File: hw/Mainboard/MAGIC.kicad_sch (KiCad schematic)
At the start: 21 parts, among them SW1 RESET, SW4 NMI, U18 SN74LVC4245APWR, U19 SN74LVC4245APWR, U20 SN74LVC4245APWR

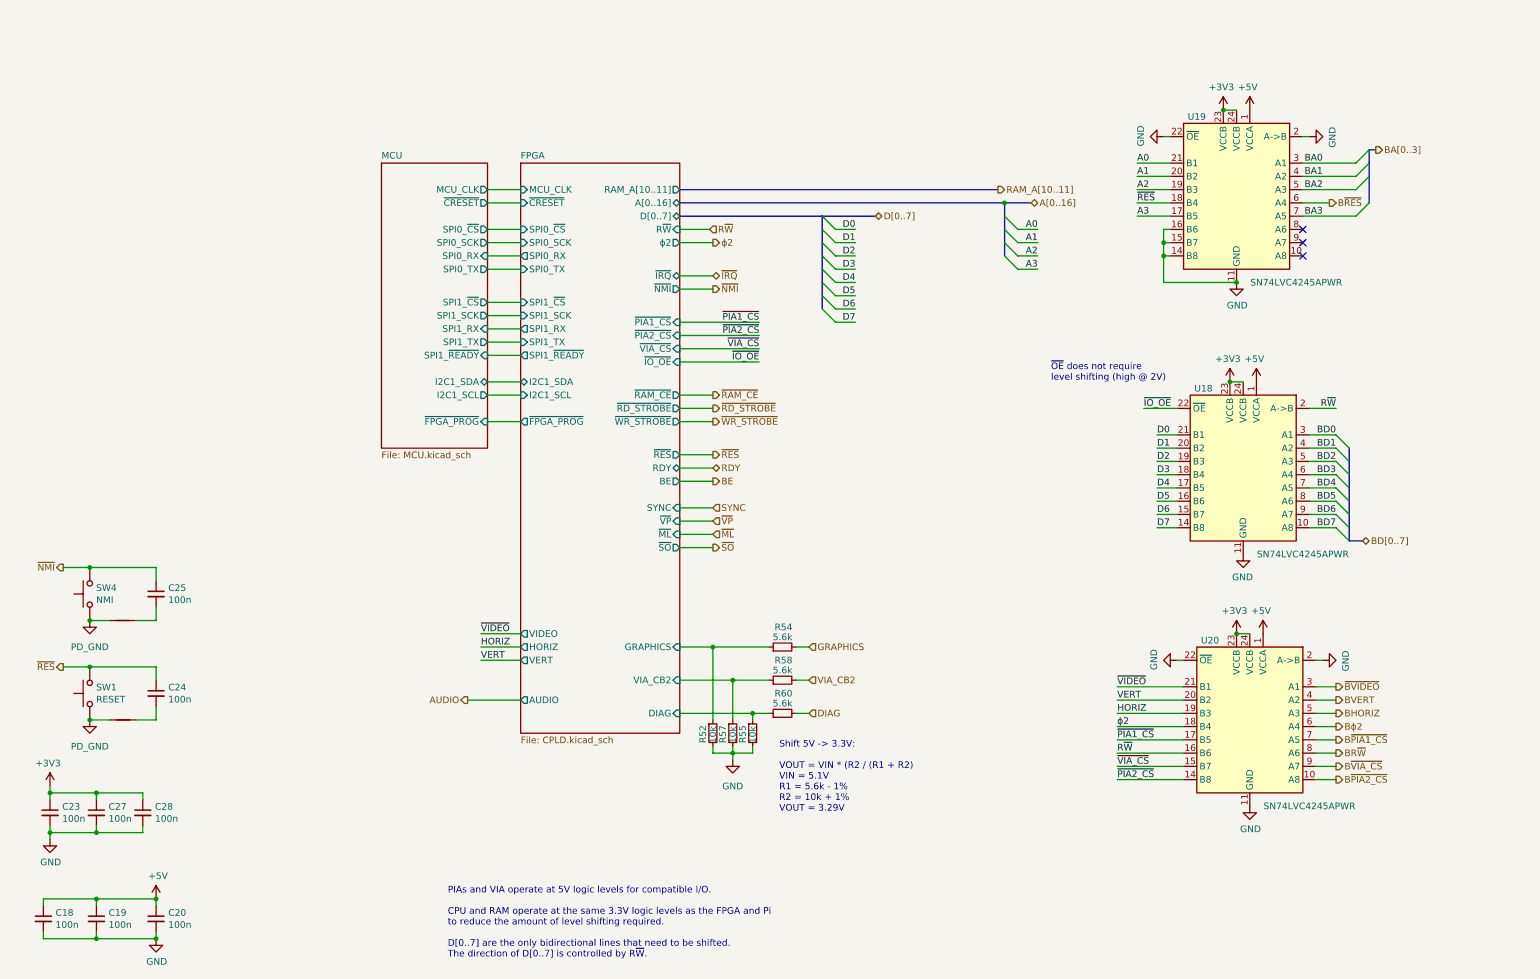
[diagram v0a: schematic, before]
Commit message: hw: wip
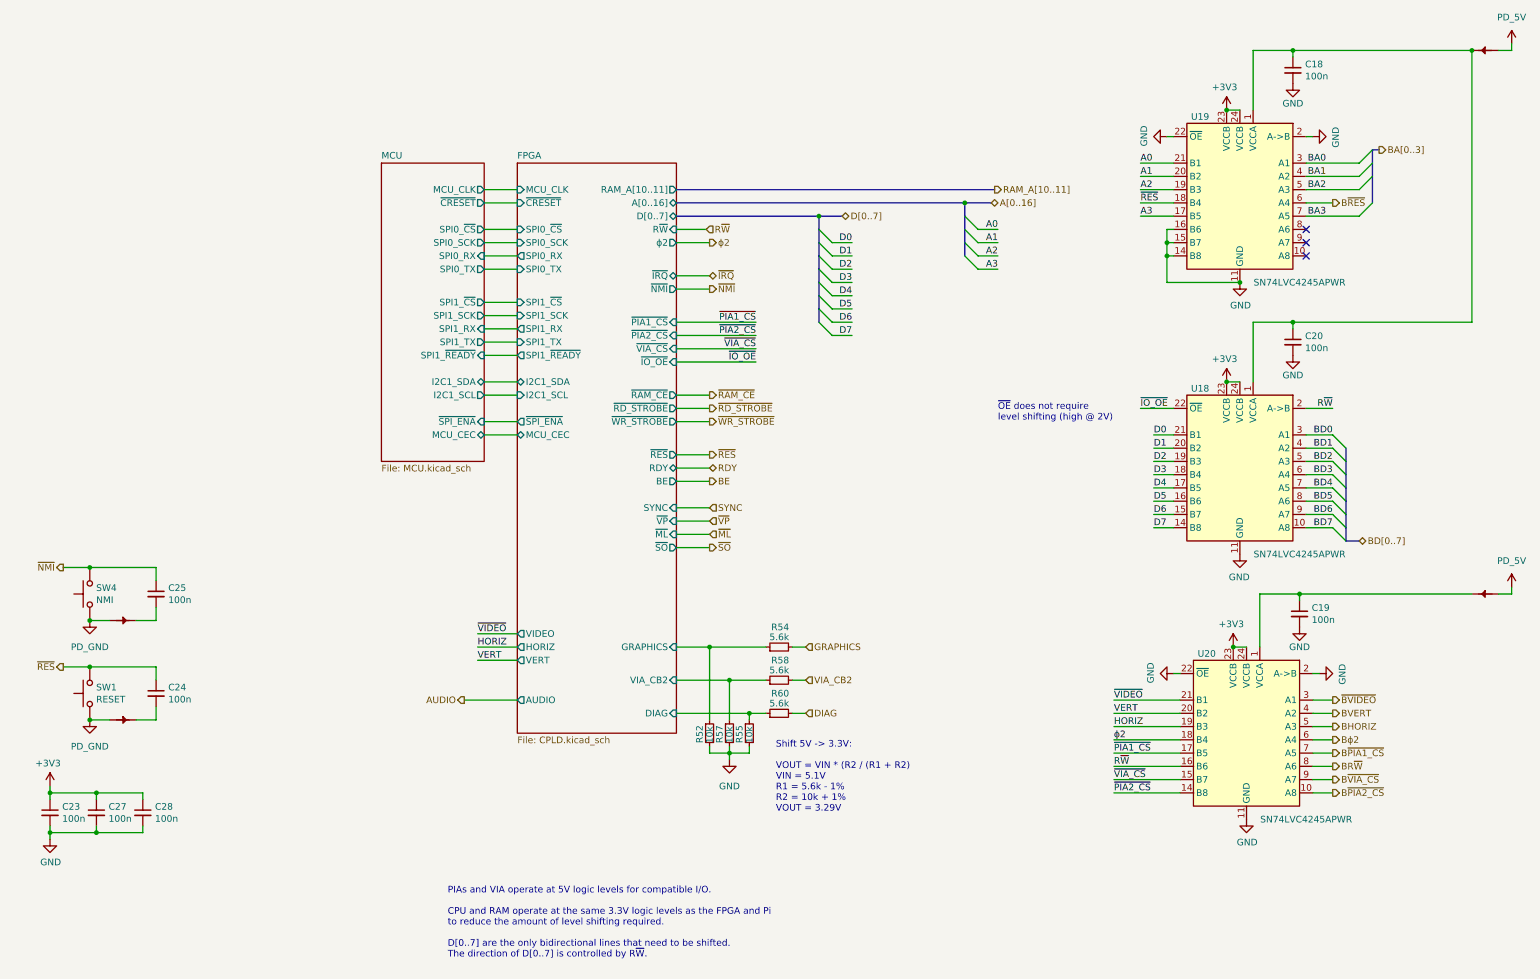
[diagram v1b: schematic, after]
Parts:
- added NT32, NT36: +5V, PET:NetTie-2_SMD_Pad_1.6_to_0.4mm, symbol PET:PowerTie_2
- NT22, NT23: symbol Device:NetTie_2 -> PET:PowerTie_2
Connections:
- net +5V: no longer names the net of C18.1, C20.1, U18.1 (VCCA), U19.1 (VCCA)
- net +5V: now also NT32.2; no longer C19.1, U20.1 (VCCA)
- new net: C19.1, NT36.2, U20.1 (VCCA)
- new net PD_5V: NT32.1, NT36.1
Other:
- sheet FPGA ports: added MCU_CEC, ~{SPI_ENA}; removed ~{FPGA_PROG}
- sheet MCU ports: added MCU_CEC, ~{SPI_ENA}; removed ~{FPGA_PROG}
- moved on the sheet: C18, C19, C20, R52, R54, R55, R57, R58, R60, U18, U19, U20
